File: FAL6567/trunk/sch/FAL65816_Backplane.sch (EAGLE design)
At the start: 28 parts, among them IC1 LM556D, IC2 74LS06D, IC3 74LVC74D

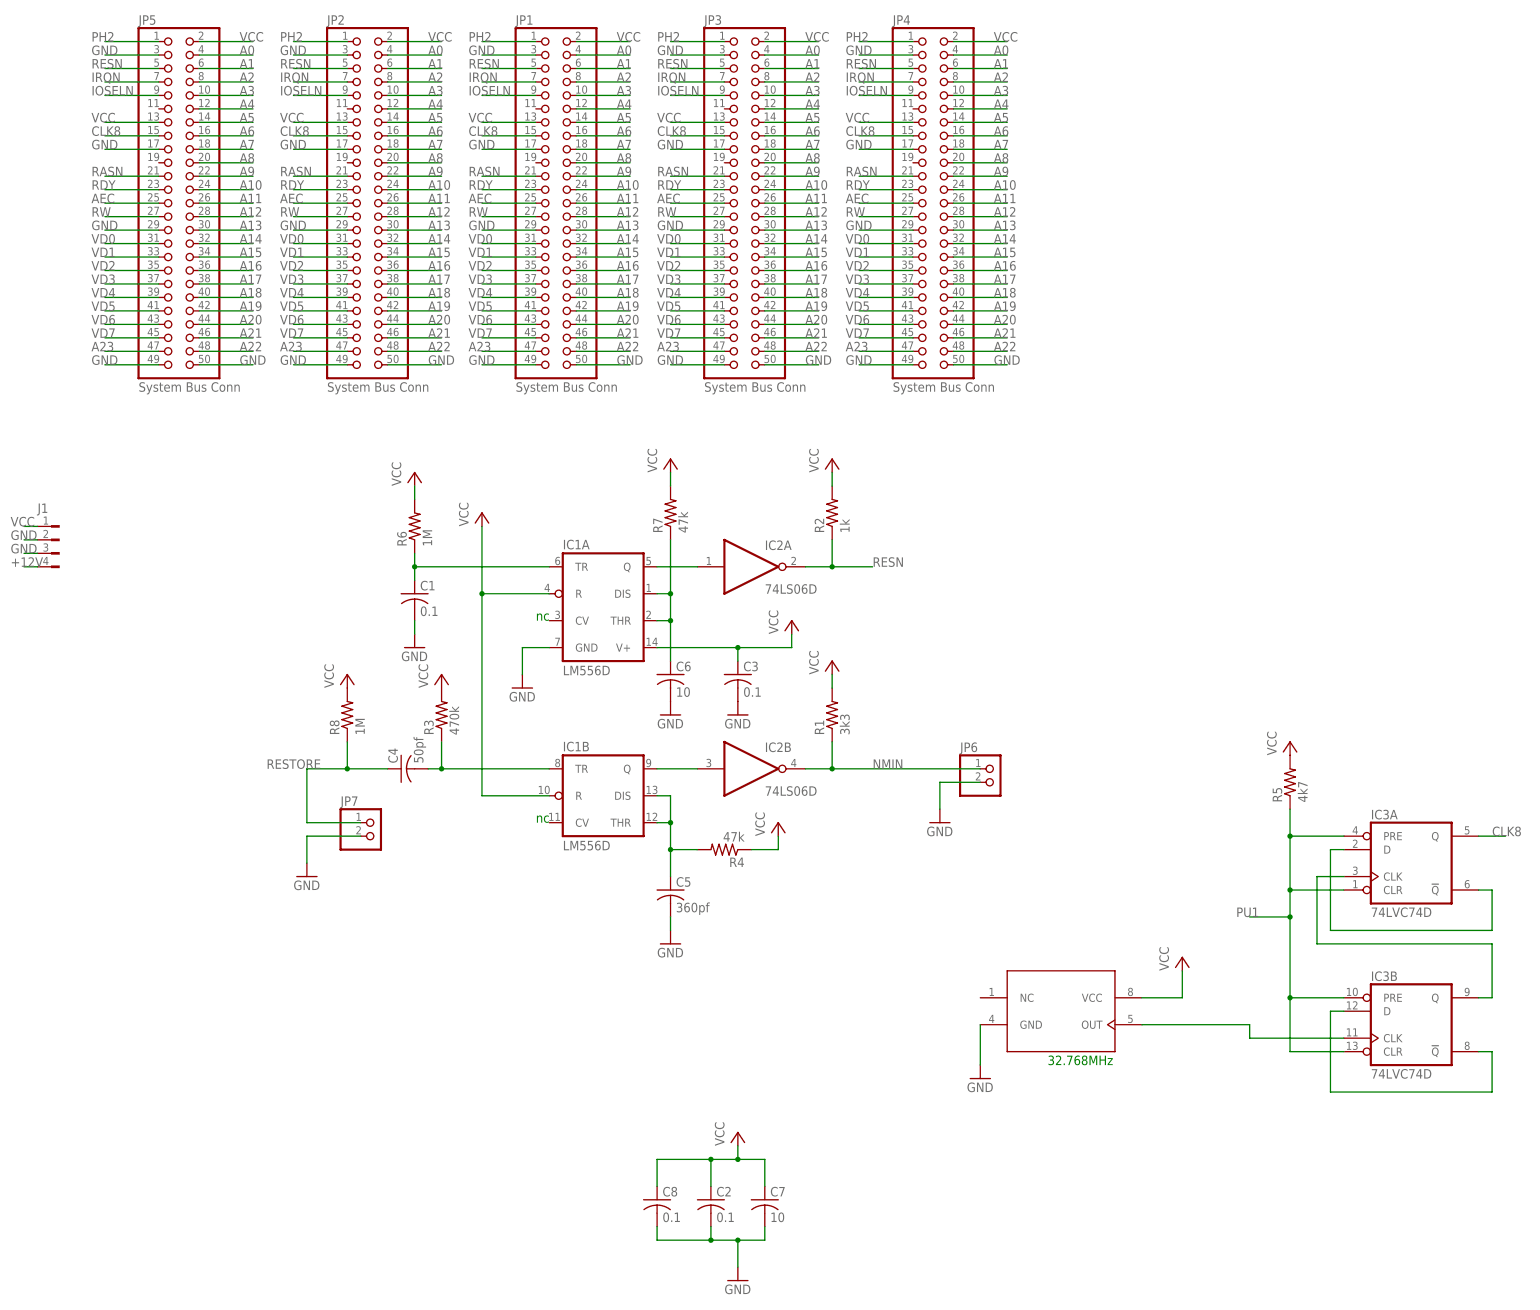
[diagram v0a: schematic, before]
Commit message: FAL65816 - update
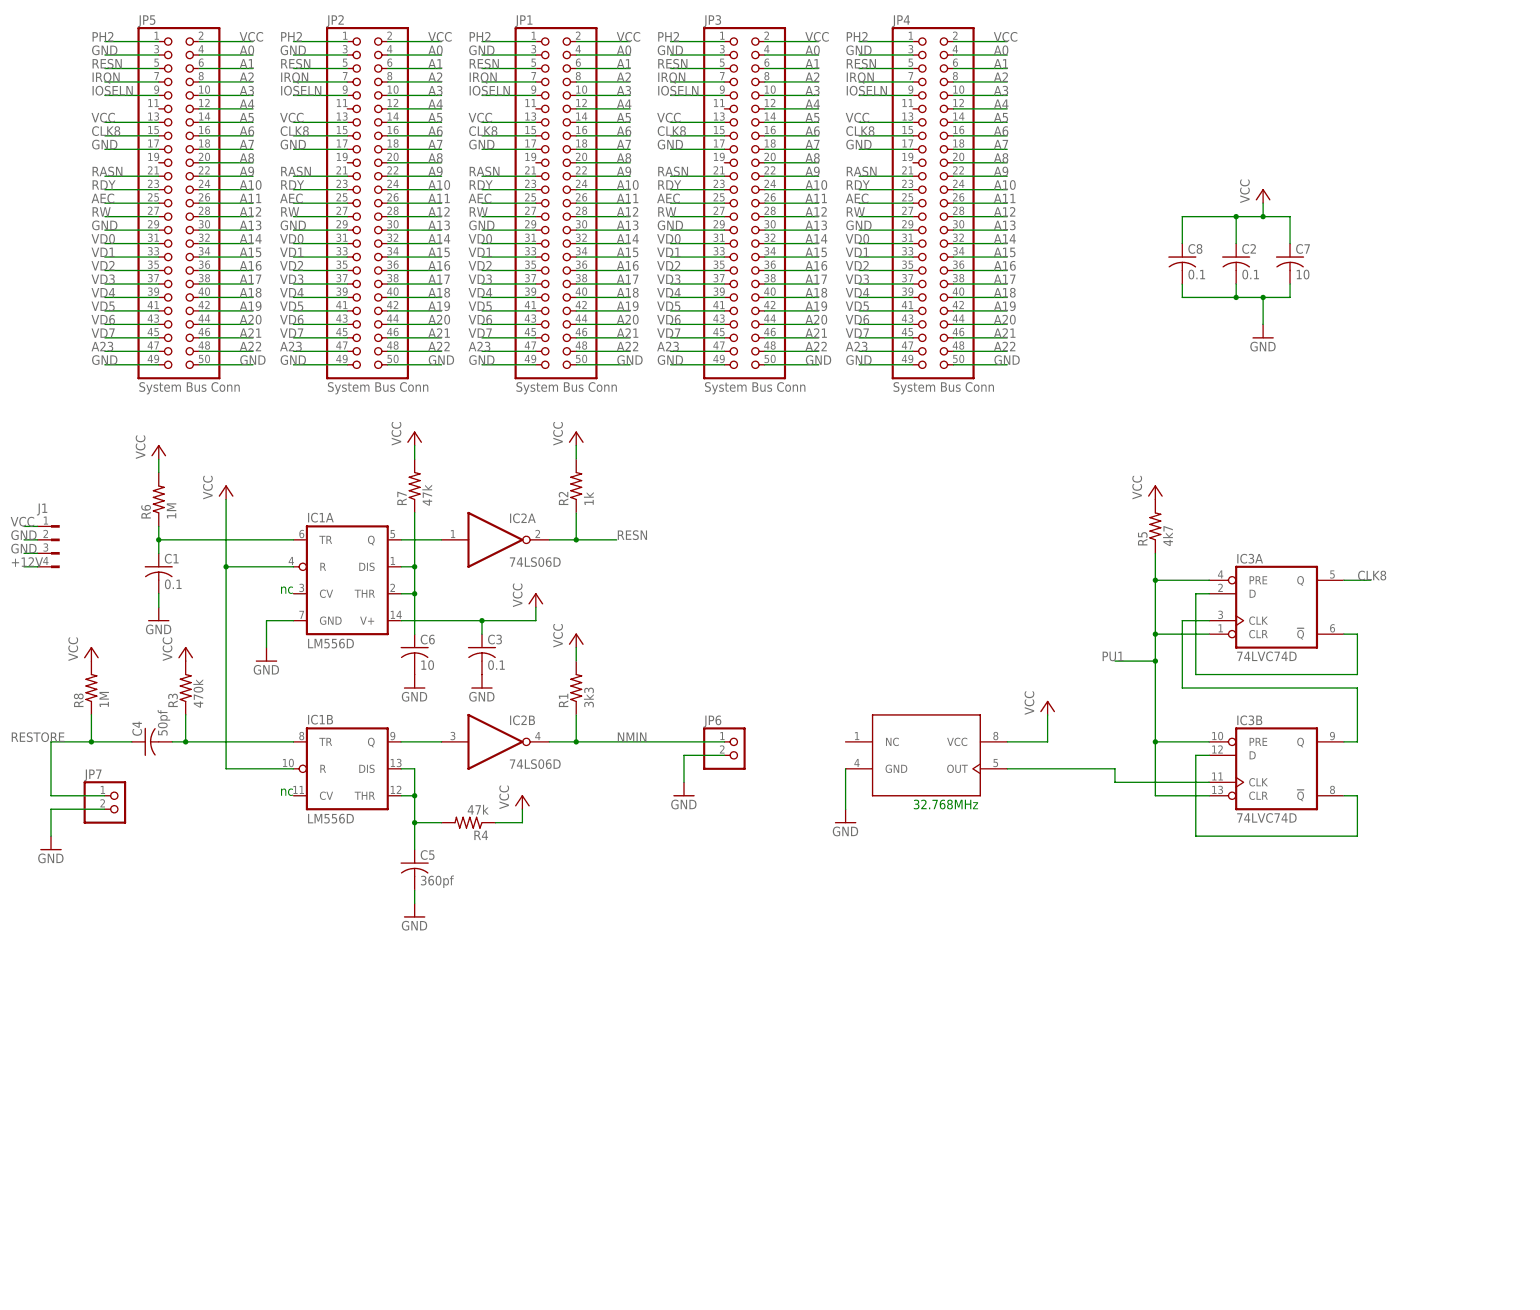
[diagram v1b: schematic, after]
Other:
- moved on the sheet: C1, C2, C3, C4, C5, C6, C7, C8, IC1A, IC1B, IC2A, IC2B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
